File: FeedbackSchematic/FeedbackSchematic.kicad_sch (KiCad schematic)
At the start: 3 parts

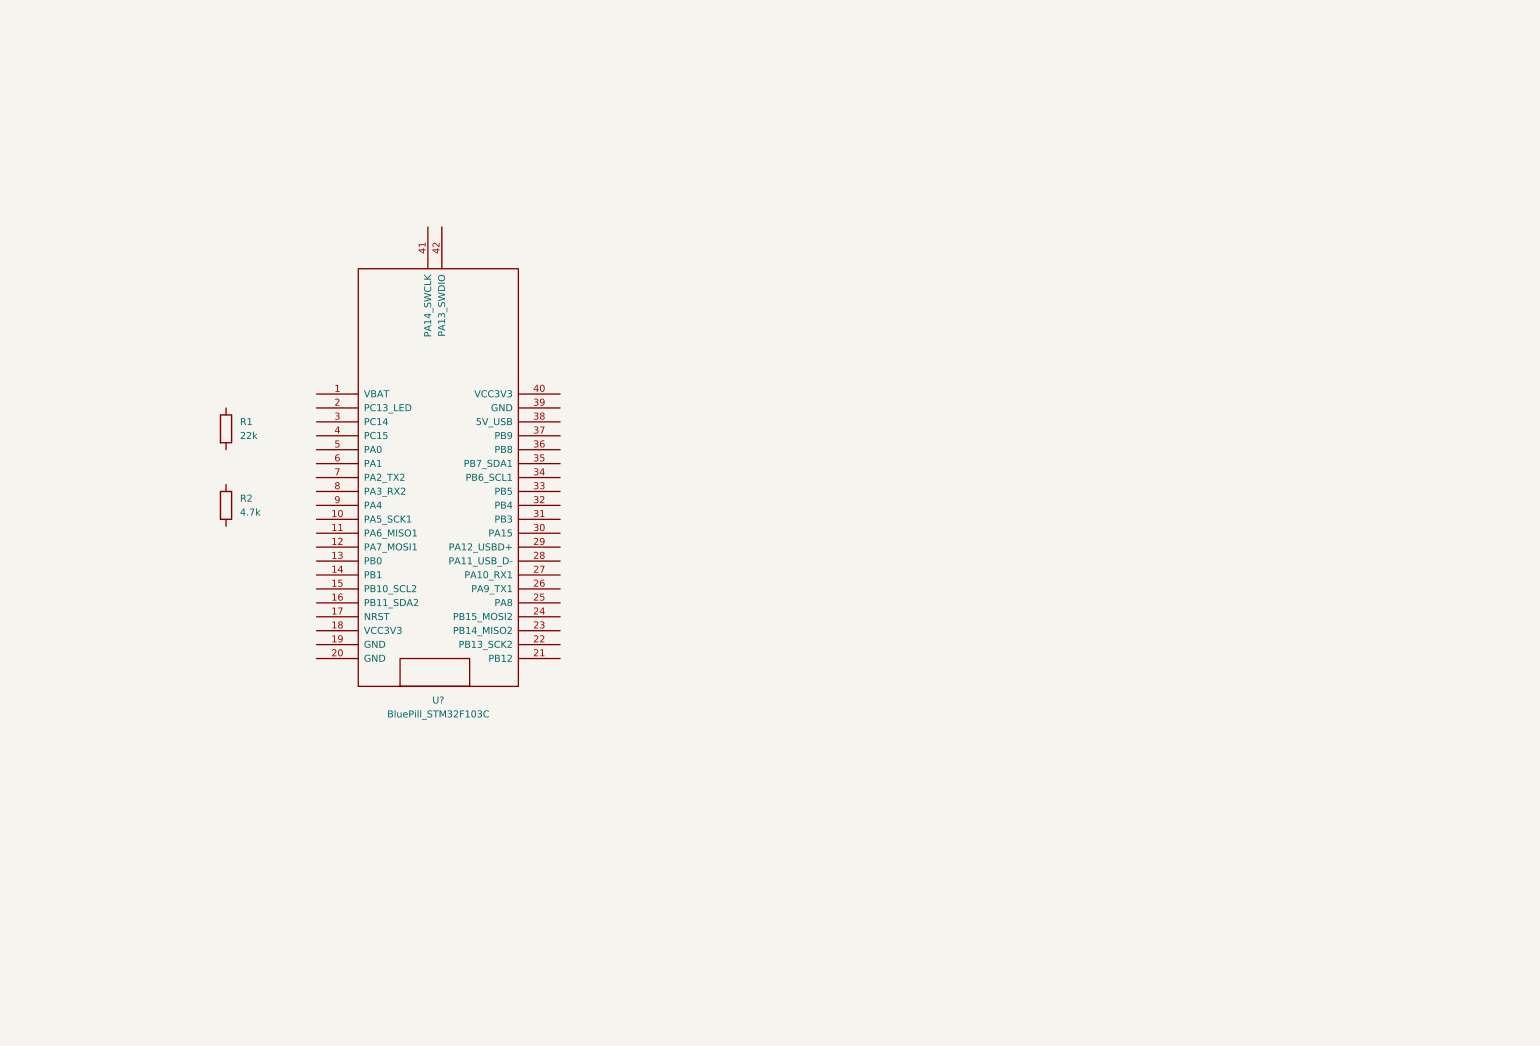
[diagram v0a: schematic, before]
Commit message: invert pin read and finish schematic
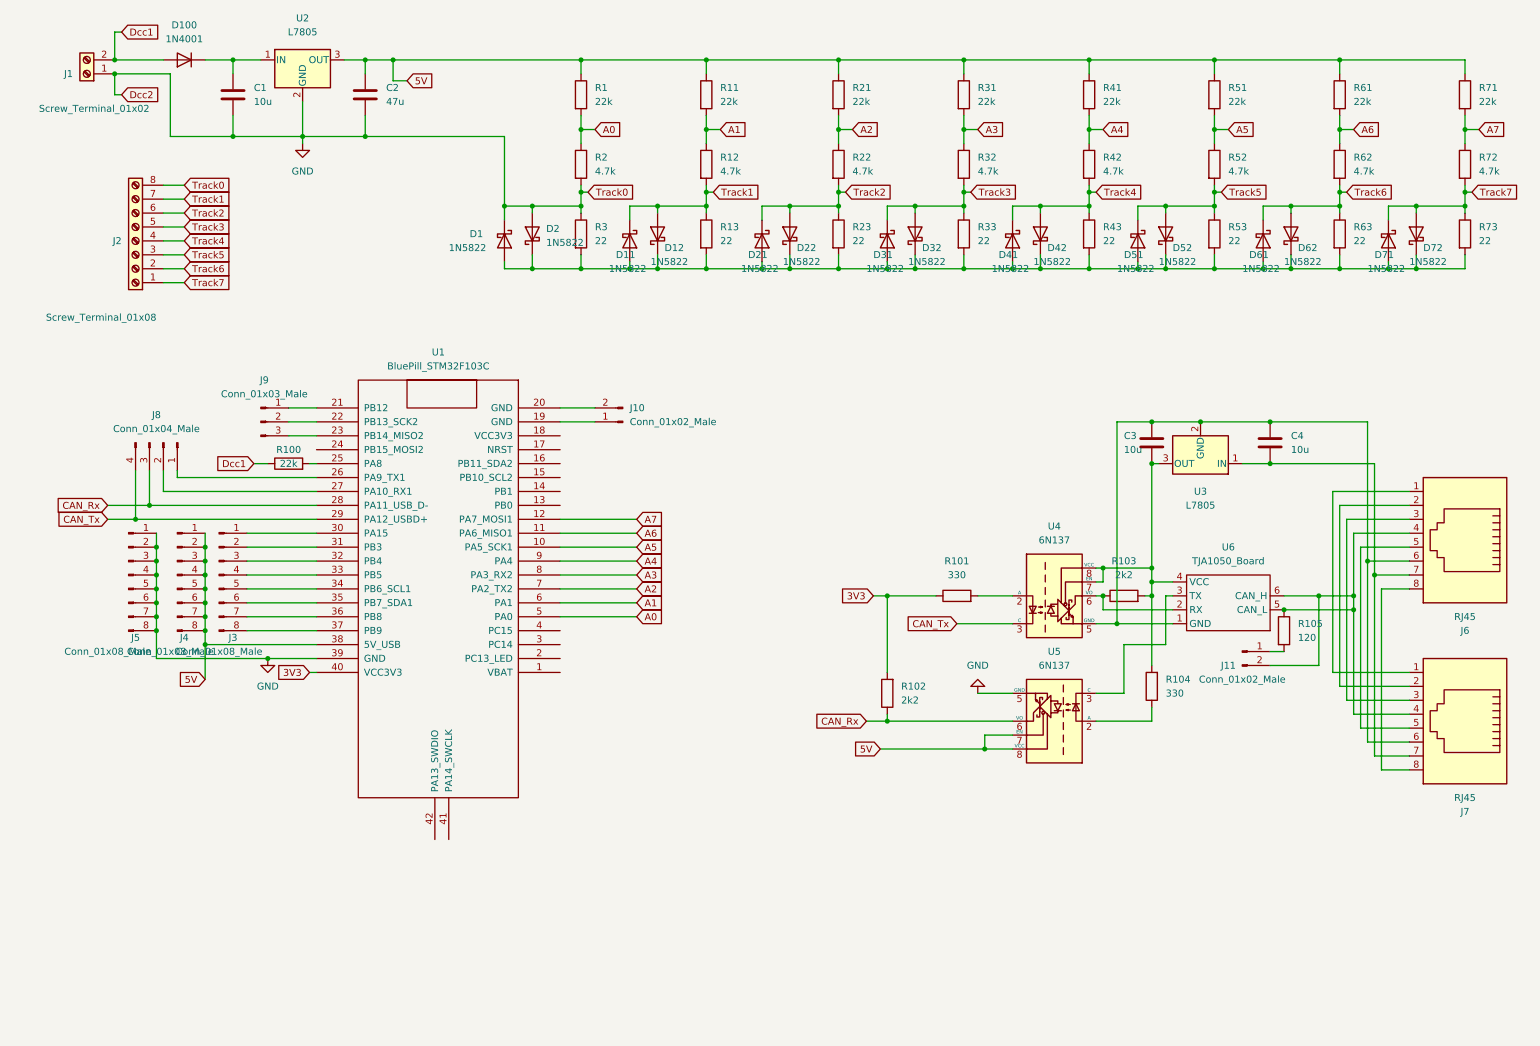
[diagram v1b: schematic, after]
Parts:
- added C1, C3, C4: 10u, symbol Device:C
- added C2: 47u, symbol Device:C
- added D1, D11, D12, D2, D21, D22, D31, D32, D41, D42, D51, D52, D61, D62, D71, D72: 1N5822, Diode_THT:D_DO-201AD_P15.24mm_Horizontal, symbol Diode:1N5822
- added D100: 1N4001, Diode_THT:D_DO-41_SOD81_P10.16mm_Horizontal, symbol Diode:1N4001
- added J1: Screw_Terminal_01x02, symbol Connector:Screw_Terminal_01x02
- added J10, J11: Conn_01x02_Male, symbol Connector:Conn_01x02_Male
- added J2: Screw_Terminal_01x08, symbol Connector:Screw_Terminal_01x08
- added J3, J4, J5: Conn_01x08_Male, symbol Connector:Conn_01x08_Male
- added J6, J7: RJ45, symbol Connector:RJ45
- added J8: Conn_01x04_Male, symbol Connector:Conn_01x04_Male
- added J9: Conn_01x03_Male, symbol Connector:Conn_01x03_Male
- added R100, R11, R21, R31, R41, R51, R61, R71: 22k, symbol Device:R
- added R101, R104: 330, symbol Device:R
- added R102, R103: 2k2, symbol Device:R
- added R105: 120, symbol Device:R
- added R12, R22, R32, R42, R52, R62, R72: 4.7k, symbol Device:R
- added R13, R23, R3, R33, R43, R53, R63, R73: 22, symbol Device:R
- added U2, U3: L7805, symbol Regulator_Linear:L7805
- added U4, U5: 6N137, Package_DIP:DIP-8_W7.62mm, symbol Isolator:6N137
- added U6: TJA1050_Board, symbol Symbols_Marcel:TJA1050_Board
- gave numbers to parts that had none: 1
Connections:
- net A5: now reaches U1.10 (PA5_SCK1)
- net A5: now also R51.2, R52.1
- net A6: now reaches U1.11 (PA6_MISO1)
- net A6: now also R61.2, R62.1
- net A7: now reaches U1.12 (PA7_MOSI1)
- net A7: now also R71.2, R72.1
- net at U1.19 (GND): now also J10.1 (Pin_1)
- net at U1.20 (GND): now also J10.2 (Pin_2)
- net at U1.21 (PB12): now also J9.1 (Pin_1)
- net at U1.22 (PB13_SCK2): now also J9.2 (Pin_2)
- net at U1.23 (PB14_MISO2): now also J9.3 (Pin_3)
- net at U1.25 (PA8): now also R100.2
- net at U1.26 (PA9_TX1): now also J8.1 (Pin_1)
- net at U1.27 (PA10_RX1): now also J8.2 (Pin_2)
- net CAN_Rx: now reaches U1.28 (PA11_USB_D-)
- net CAN_Rx: now also J8.3 (Pin_3), R102.1, U5.6 (VO)
- net CAN_Tx: now reaches U1.29 (PA12_USBD+)
- net CAN_Tx: now also J8.4 (Pin_4), U4.3 (C)
- net at U1.30 (PA15): now also J3.1 (Pin_1)
- net at U1.31 (PB3): now also J3.2 (Pin_2)
- net at U1.32 (PB4): now also J3.3 (Pin_3)
- net at U1.33 (PB5): now also J3.4 (Pin_4)
- net at U1.34 (PB6_SCL1): now also J3.5 (Pin_5)
- net at U1.35 (PB7_SDA1): now also J3.6 (Pin_6)
- net at U1.36 (PB8): now also J3.7 (Pin_7)
- net at U1.37 (PB9): now also J3.8 (Pin_8)
- net 5V: now reaches U1.38 (5V_USB)
- net 5V: now also R1.1, C2.1, J4.1 (Pin_1), J4.2 (Pin_2), J4.3 (Pin_3), J4.4 (Pin_4), J4.5 (Pin_5), J4.6 (Pin_6), J4.7 (Pin_7), J4.8 (Pin_8), R11.1, R21.1, R31.1, R41.1, R51.1, R61.1, R71.1, U2.3 (OUT), U5.7 (EN), U5.8 (VCC)
- net GND: now reaches U1.39 (GND)
- net GND: now also R2.2, C1.2, C2.2, D1.1 (K), D2.2 (A), J1.1 (Pin_1), J2.8 (Pin_8), J5.1 (Pin_1), J5.2 (Pin_2), J5.3 (Pin_3), J5.4 (Pin_4), J5.5 (Pin_5), J5.6 (Pin_6), J5.7 (Pin_7), J5.8 (Pin_8), R3.1, U2.2 (GND), U5.5 (GND)
- net 3V3: now reaches U1.40 (VCC3V3)
- net 3V3: now also R101.1, R102.2
- net A0: now reaches U1.5 (PA0)
- net A0: now also R1.2, R2.1
- net A1: now reaches U1.6 (PA1)
- net A1: now also R11.2, R12.1
- net A2: now reaches U1.7 (PA2_TX2)
- net A2: now also R21.2, R22.1
- net A3: now reaches U1.8 (PA3_RX2)
- net A3: now also R31.2, R32.1
- net A4: now reaches U1.9 (PA4)
- net A4: now also R41.2, R42.1
- new net: R101.2, U4.2 (A)
- new net: C3.2, C4.1, J6.6, J7.6, U3.2 (GND), U4.5 (GND), U6.1 (GND)
- new net: R103.1, U4.6 (VO), U6.2 (RX)
- new net: C3.1, R103.2, R104.2, U3.3 (OUT), U4.7 (EN), U4.8 (VCC), U6.4 (VCC)
- new net: D1.2 (A), D11.2 (A), D12.1 (K), D2.1 (K), D21.2 (A), D22.1 (K), D31.2 (A), D32.1 (K), D41.2 (A), D42.1 (K), D51.2 (A), D52.1 (K), D61.2 (A), D62.1 (K), D71.2 (A), D72.1 (K), R13.2, R23.2, R3.2, R33.2, R43.2, R53.2, R63.2, R73.2
- new net: C4.2, J6.7, J7.7, U3.1 (IN)
- new net: J6.1, J7.1
- new net: J6.2, J7.2
- new net: J6.3, J7.3
- new net: J11.2 (Pin_2), J6.4, J7.4, R105.1, U6.5 (CAN_L), U6.6 (CAN_H)
- new net: J6.5, J7.5
- new net: J6.8, J7.8
- new net: U5.3 (C), U6.3 (TX)
- new net: R104.1, U5.2 (A)
- new net: J11.1 (Pin_1), R105.2
- new net: C1.1, D100.1 (K), U2.1 (IN)
- new net Dcc1: D100.2 (A), J1.2 (Pin_2), R100.1
- new net Track1: D11.1 (K), D12.2 (A), J2.7 (Pin_7), R12.2, R13.1
- new net Track2: D21.1 (K), D22.2 (A), J2.6 (Pin_6), R22.2, R23.1
- new net Track3: D31.1 (K), D32.2 (A), J2.5 (Pin_5), R32.2, R33.1
- new net Track4: D41.1 (K), D42.2 (A), J2.4 (Pin_4), R42.2, R43.1
- new net Track5: D51.1 (K), D52.2 (A), J2.3 (Pin_3), R52.2, R53.1
- new net Track6: D61.1 (K), D62.2 (A), J2.2 (Pin_2), R62.2, R63.1
- new net Track7: D71.1 (K), D72.2 (A), J2.1 (Pin_1), R72.2, R73.1
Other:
- moved on the sheet: R1, R2, U1

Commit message: Updated schematics
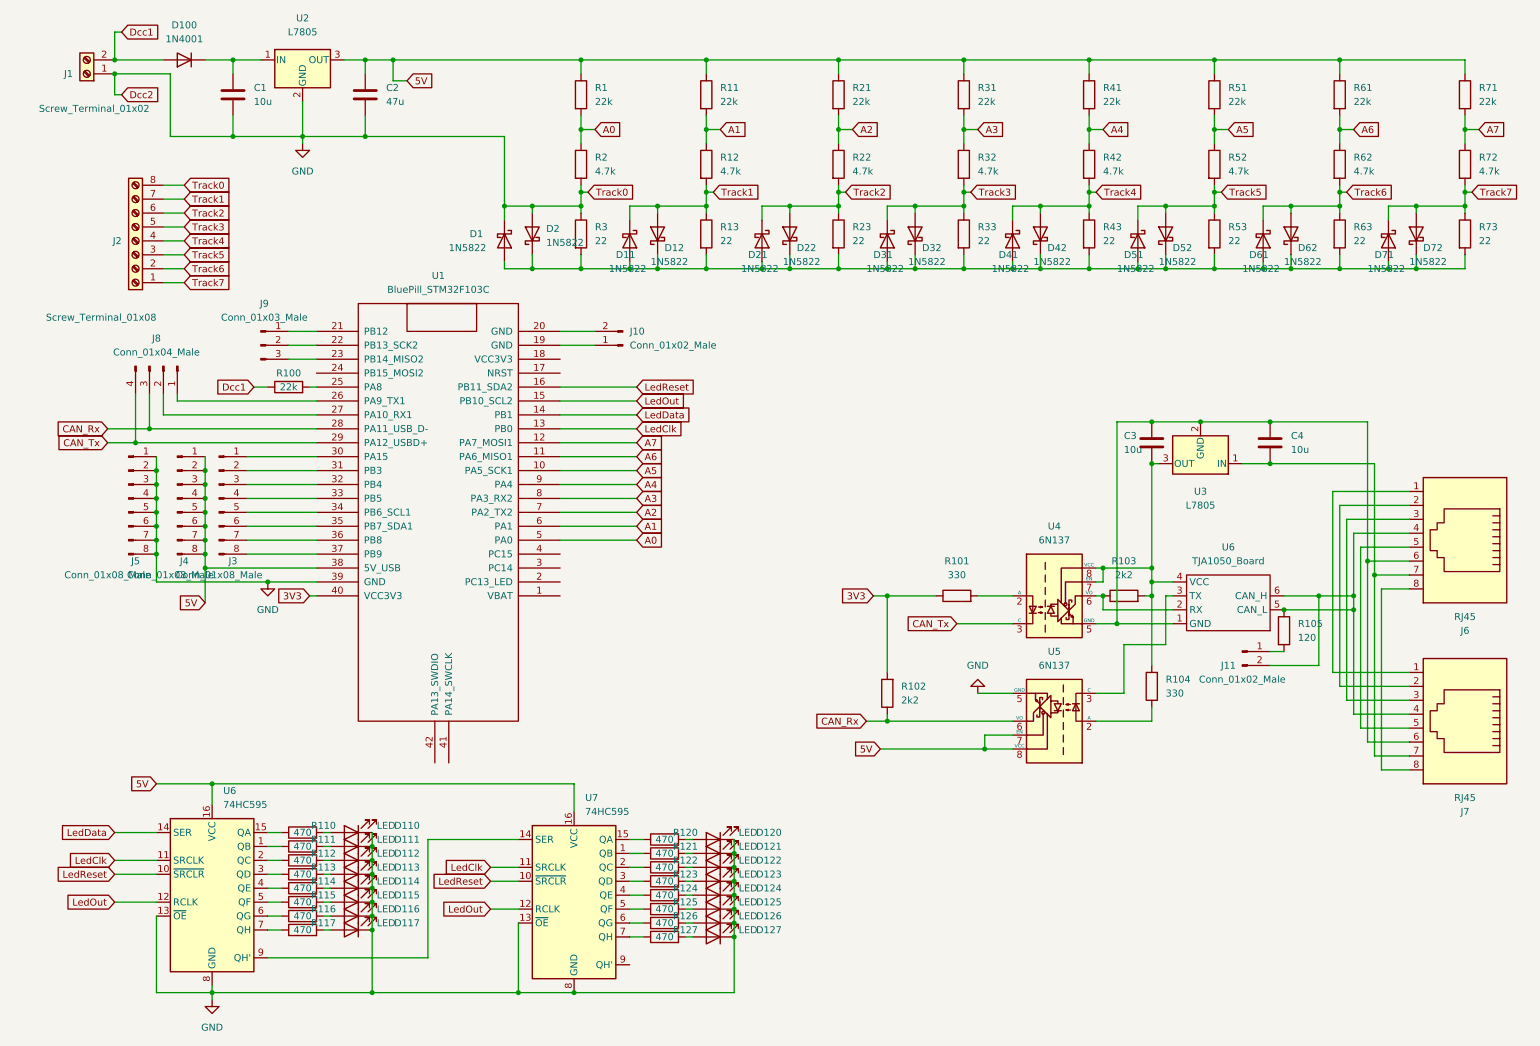
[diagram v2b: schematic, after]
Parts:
- added D110, D111, D112, D113, D114, D115, D116, D117, D120, D121, D122, D123, D124, D125, D126, D127: LED, symbol Device:LED
- added R110, R111, R112, R113, R114, R115, R116, R117, R120, R121, R122, R123, R124, R125, R126, R127: 470, symbol Device:R
- added U6, U7: 74HC595, symbol 74xx:74HC595
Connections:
- net 5V: now also U6.16 (VCC), U7.16 (VCC)
- net GND: now also D110.1 (K), D111.1 (K), D112.1 (K), D113.1 (K), D114.1 (K), D115.1 (K), D116.1 (K), D117.1 (K), D120.1 (K), D121.1 (K), D122.1 (K), D123.1 (K), D124.1 (K), D125.1 (K), D126.1 (K), D127.1 (K), U6.13 (~{OE}), U6.8 (GND), U7.13 (~{OE}), U7.8 (GND)
- net LedClk: now reaches U1.13 (PB0)
- net LedClk: now also U6.11 (SRCLK), U7.11 (SRCLK)
- net LedData: now reaches U1.14 (PB1)
- net LedData: now also U6.14 (SER)
- net LedOut: now reaches U1.15 (PB10_SCL2)
- net LedOut: now also U6.12 (RCLK), U7.12 (RCLK)
- net LedReset: now reaches U1.16 (PB11_SDA2)
- net LedReset: now also U6.10 (~{SRCLR}), U7.10 (~{SRCLR})
- new net: R113.1, U6.3 (QD)
- new net: D113.2 (A), R113.2
- new net: R111.1, U6.1 (QB)
- new net: R110.1, U6.15 (QA)
- new net: R112.1, U6.2 (QC)
- new net: R114.1, U6.4 (QE)
- new net: R115.1, U6.5 (QF)
- new net: R116.1, U6.6 (QG)
- new net: R117.1, U6.7 (QH)
- new net: U6.9 (QH'), U7.14 (SER)
- new net: R123.1, U7.3 (QD)
- new net: D123.2 (A), R123.2
- new net: R121.1, U7.1 (QB)
- new net: R120.1, U7.15 (QA)
- new net: R122.1, U7.2 (QC)
- new net: R124.1, U7.4 (QE)
- new net: R125.1, U7.5 (QF)
- new net: R126.1, U7.6 (QG)
- new net: R127.1, U7.7 (QH)
- new net: D110.2 (A), R110.2
- new net: D126.2 (A), R126.2
- new net: D116.2 (A), R116.2
- new net: D114.2 (A), R114.2
- new net: D112.2 (A), R112.2
- new net: D120.2 (A), R120.2
- new net: D124.2 (A), R124.2
- new net: D111.2 (A), R111.2
- new net: D122.2 (A), R122.2
- new net: D125.2 (A), R125.2
- new net: D117.2 (A), R117.2
- new net: D121.2 (A), R121.2
- new net: D127.2 (A), R127.2
- new net: D115.2 (A), R115.2
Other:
- moved on the sheet: J10, J3, J4, J5, J8, J9, R100, U1
